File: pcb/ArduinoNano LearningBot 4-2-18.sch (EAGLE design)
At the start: 21 parts

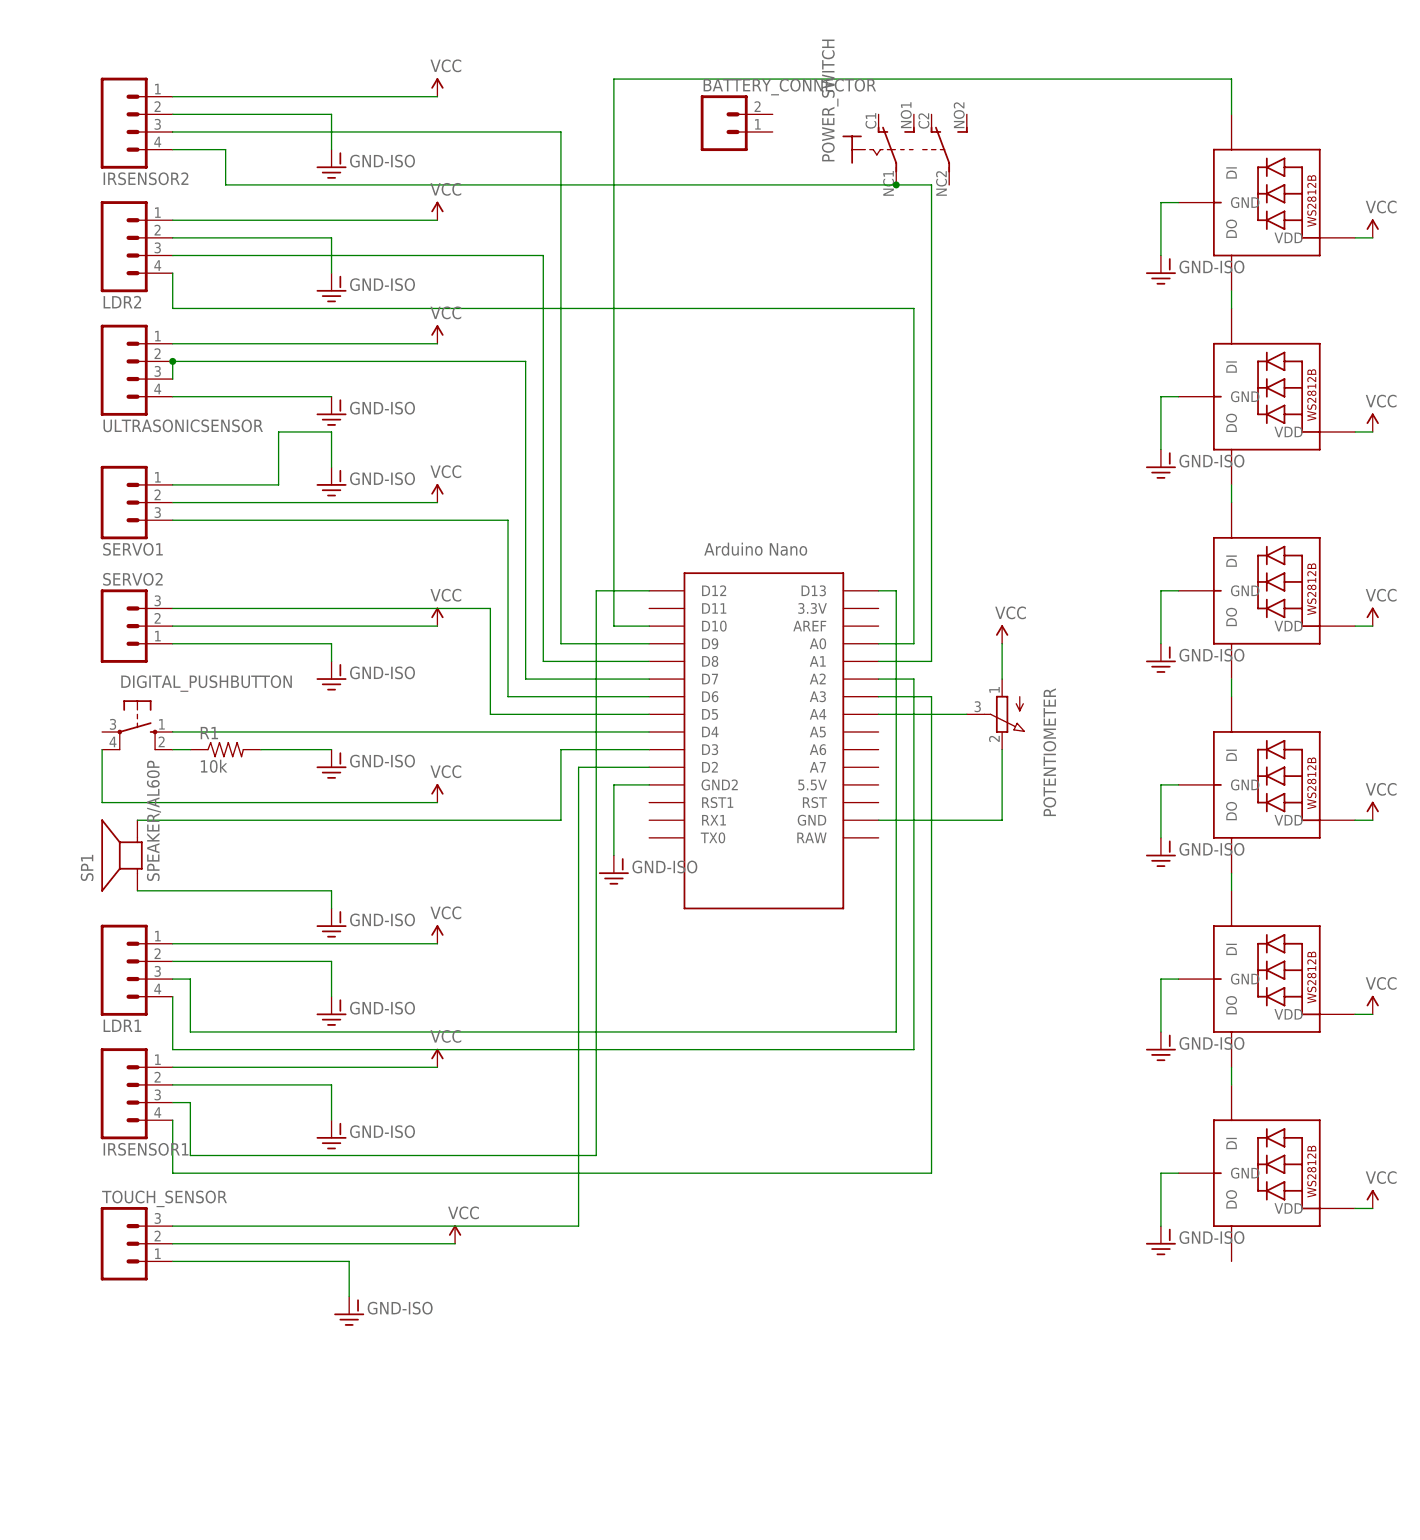
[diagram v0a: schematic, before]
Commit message: yes
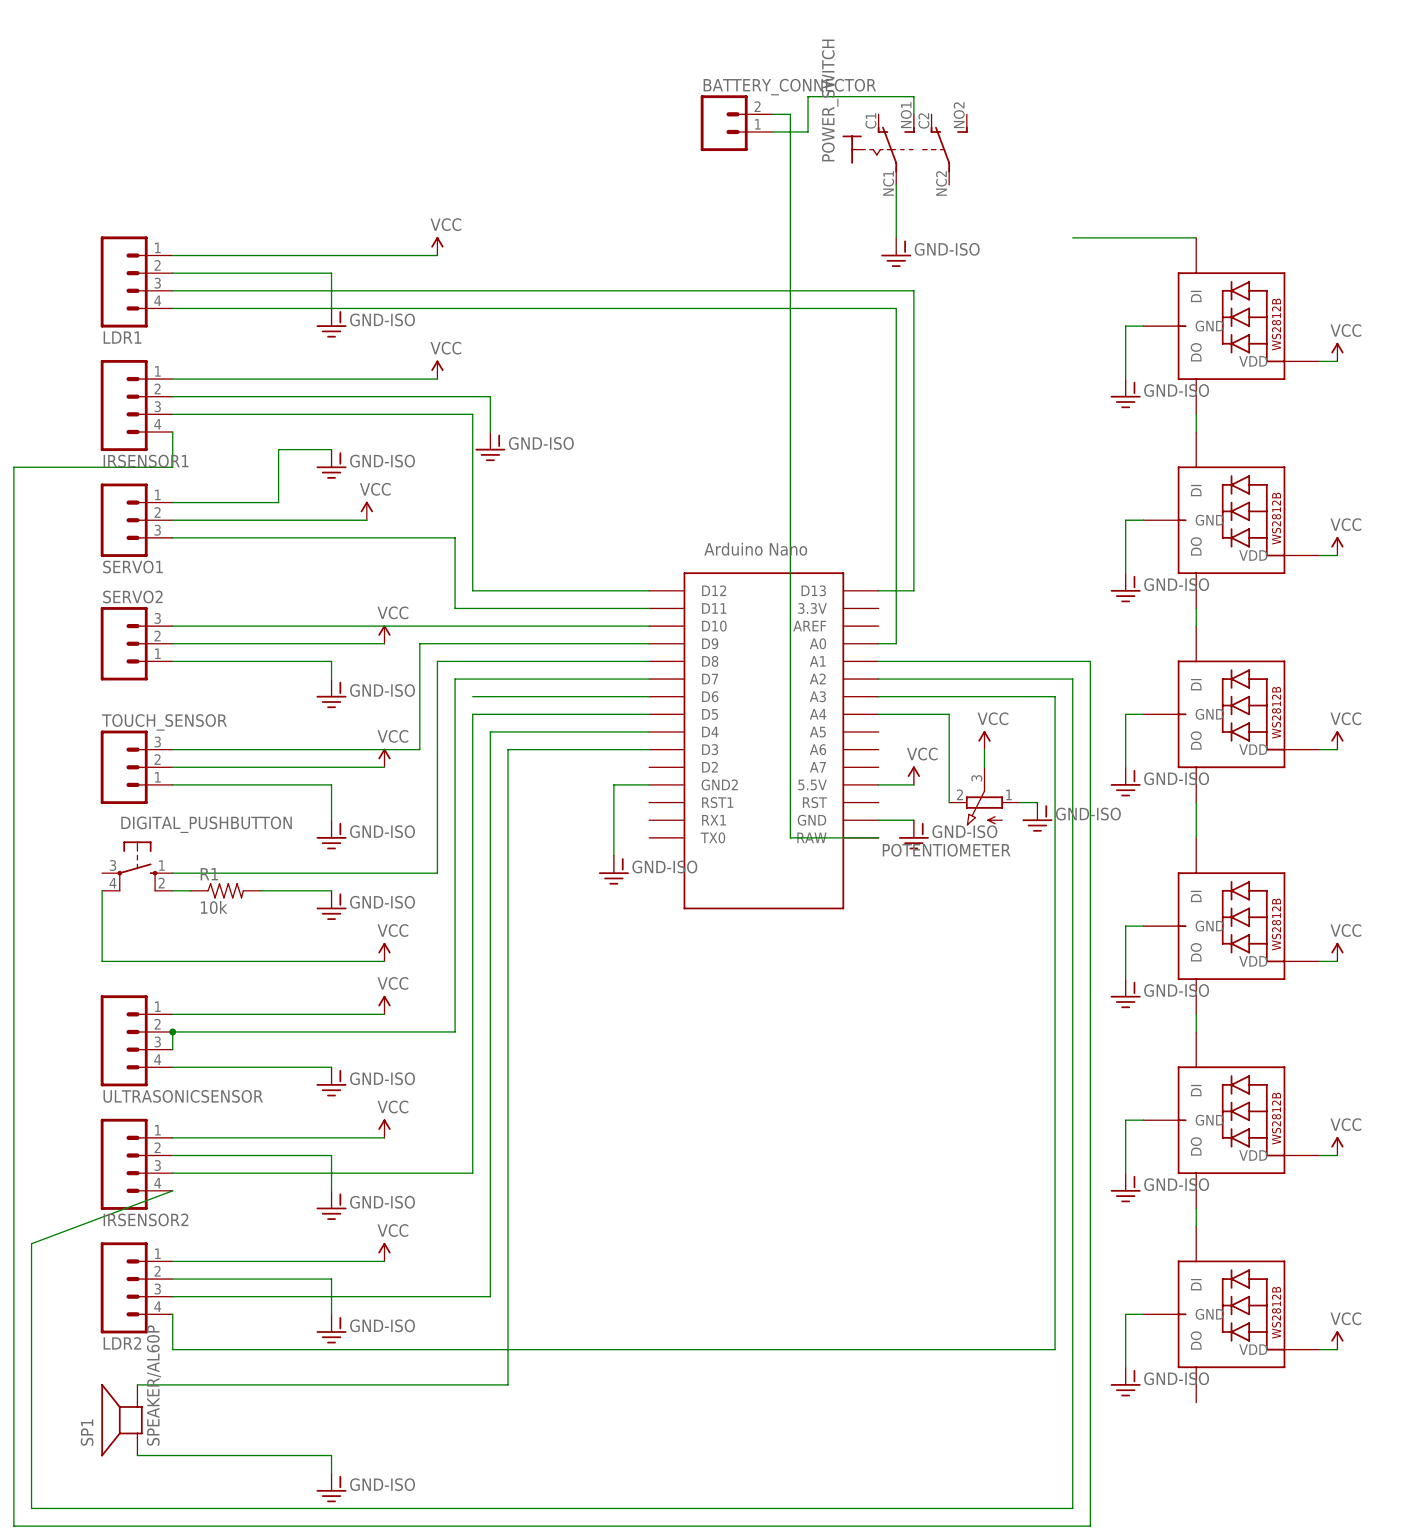
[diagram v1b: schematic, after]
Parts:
- removed LED1, LED2, LED3, LED4, LED5, LED6: WS2812B5050, adafruit:WS2812B5050
- added LED-1, LED-2, LED-3, LED-4, LED-5, LED-6: WS2812B5050, adafruit:WS2812B5050
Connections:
- removed net DIGITAL_PUSHBUTTON_PIN: DIGITAL_PUSHBUTTON.S, U$1.D4
- removed net N$5: LED4.DO, LED6.DI
- removed net N$7: POTENTIOMETER.S, U$1.A4
- new net BUTTON: DIGITAL_PUSHBUTTON.S, U$1.D8
- new net LED-1: LED-1.DI, U$1.D6
- new net N$9: BATTERY_CONNECTOR.1, POWER_SWITCH1.S
- new net POTPIN: POTENTIOMETER.E, U$1.A4
- new net RAWIN: BATTERY_CONNECTOR.2, U$1.RAW
- net GND: now also LED-1.GND, LED-2.GND, LED-3.GND, LED-4.GND, LED-5.GND, LED-6.GND, POTENTIOMETER.A, POWER_SWITCH1.P; no longer LED1.GND, LED2.GND, LED3.GND, LED4.GND, LED5.GND, LED6.GND, POTENTIOMETER.E
- net IR_SENSOR1_AO: now also U$1.A1; no longer U$1.A3
- net IR_SENSOR2_AO: now also U$1.A2; no longer POWER_SWITCH1.P, U$1.A1
- net IR_SENSOR2_DO: now also U$1.D5; no longer U$1.D9
- net LDR1_AO: now also U$1.A0; no longer U$1.A2
- net LDR2_AO: now also U$1.A3; no longer U$1.A0
- net LDR2_DO: now also U$1.D4; no longer U$1.D8
- net N$1: now also LED-3.DO, LED-4.DI; no longer LED2.DI, U$1.D10
- net N$2: now also LED-4.DO, LED-5.DI; no longer LED1.DI, LED2.DO
- net N$4: now also LED-5.DO, LED-6.DI; no longer LED1.DO, LED4.DI
- net N$6: now also LED-1.DO, LED-2.DI; no longer LED3.DI, LED6.DO
- net N$8: now also LED-2.DO, LED-3.DI; no longer LED3.DO, LED5.DI
- net SERVO1_PIN: now also U$1.D11; no longer U$1.D6
- net SERVO2_PIN: now also U$1.D10; no longer U$1.D5
- net TOUCH_SENSOR: now also U$1.D9; no longer U$1.D2
- net VCC: now also LED-1.VDD, LED-2.VDD, LED-3.VDD, LED-4.VDD, LED-5.VDD, LED-6.VDD, POTENTIOMETER.S, U$1.5.5V; no longer LED1.VDD, LED2.VDD, LED3.VDD, LED4.VDD, LED5.VDD, LED6.VDD, POTENTIOMETER.A
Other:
- moved on the sheet: DIGITAL_PUSHBUTTON, IRSENSOR1, IRSENSOR2, LDR1, LDR2, POTENTIOMETER, R1, SERVO1, SERVO2, SP1, TOUCH_SENSOR, ULTRASONICSENSOR
